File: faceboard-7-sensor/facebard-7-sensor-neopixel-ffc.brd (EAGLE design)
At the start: 26 x 93.5 mm, 32 parts, among them Q1 QRE1113, Q2 QRE1113, Q3 QRE1113, Q4 QRE1113, Q5 QRE1113, Q6 QRE1113, Q7 QRE1113, U1 CD4051BE

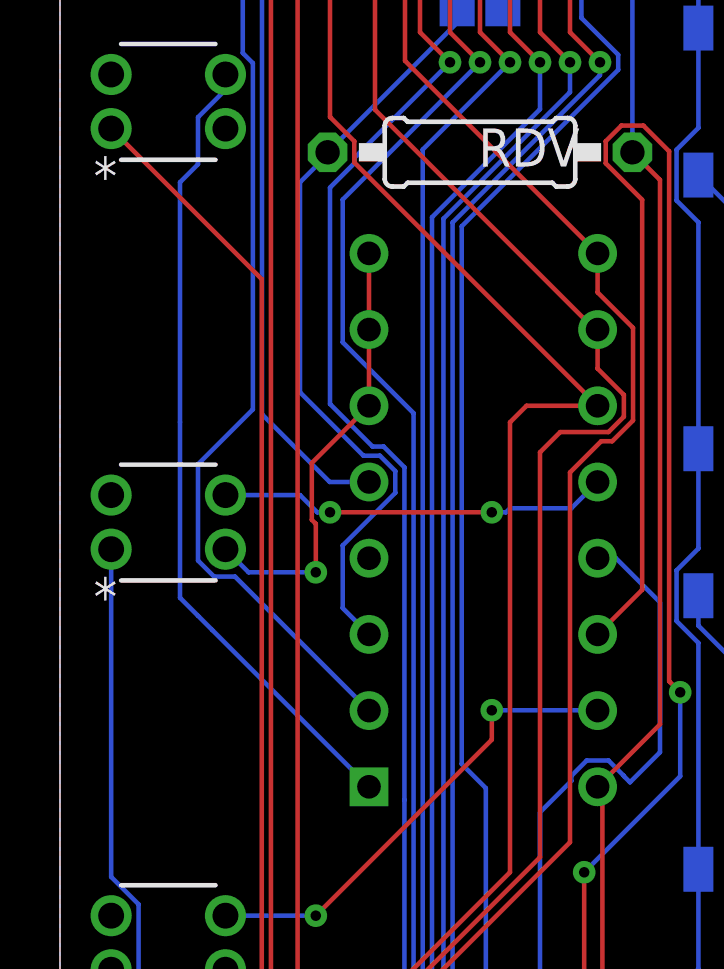
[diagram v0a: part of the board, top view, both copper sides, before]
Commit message: tidy routing
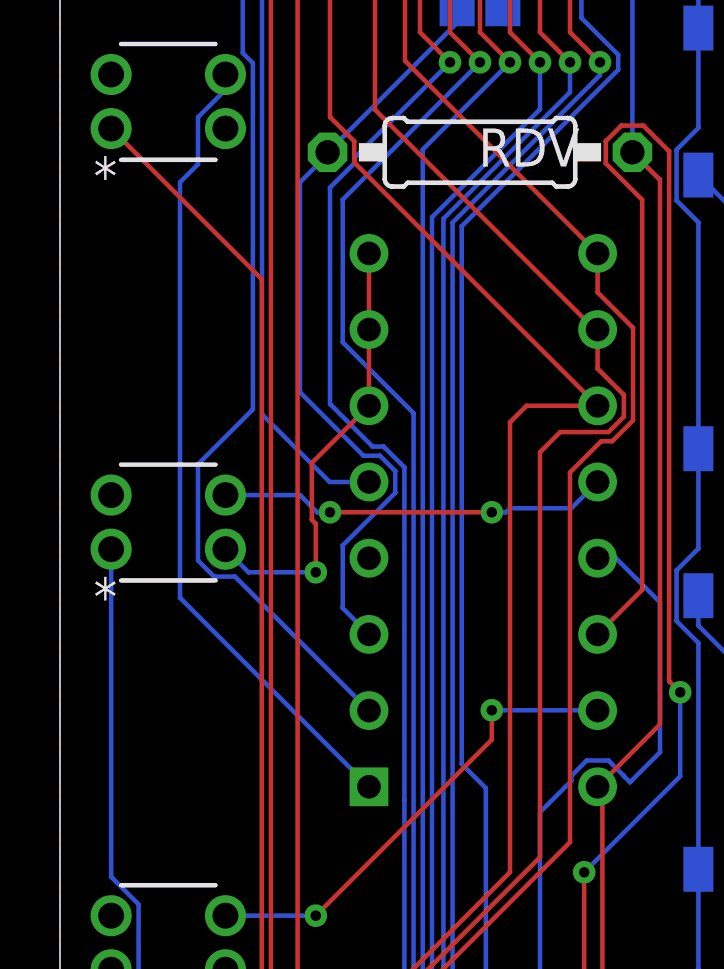
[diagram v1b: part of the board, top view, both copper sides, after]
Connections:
- net Q1SIG renamed C0
- net Q2SIG renamed C1
- net Q3SIG renamed C2
- net Q4SIG renamed C3
- net Q5SIG renamed C4
- net Q6SIG renamed C5
- net Q7SIG renamed C6
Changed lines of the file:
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@@
 <wire x1="6.7" y1="15.7" x2="7.92" y2="15.7" width="0.1524" layer="1"/>
 </signal>
-<signal name="Q1SIG">
+<signal name="C0">
 <contactref element="U1" pad="13"/>
-<contactref element="Q1" pad="3"/>
-<wire x1="5.515" y1="5.5134" x2="5.515" y2="12.515" width="0.1524" layer="16"/>
 <wire x1="5.515" y1="12.515" x2="7" y2="14" width="0.1524" layer="16"/>
 <wire x1="7" y1="14" x2="11" y2="14" width="0.1524" layer="16"/>
@@
 <wire x1="20" y1="39" x2="20" y2="44" width="0.1524" layer="16"/>
 <wire x1="20" y1="44" x2="18.53" y2="45.47" width="0.1524" layer="16"/>
+<contactref element="Q1" pad="3"/>
+<wire x1="5.515" y1="5.5134" x2="5.515" y2="12.515" width="0.1524" layer="16"/>
 </signal>
 <signal name="GND">
@@
 <wire x1="6.5356" y1="16.8156" x2="7.92" y2="18.2" width="0.1524" layer="1"/>
 </signal>
-<signal name="Q2SIG">
-<contactref element="Q2" pad="3"/>
+<signal name="C1">
 <contactref element="U1" pad="14"/>
 <via x="11" y="20.4334" extent="1-16" drill="0.35"/>
@@
 <wire x1="20.3048" y1="41.3684" x2="20.3048" y2="59.0324375" width="0.1524" layer="1"/>
 <wire x1="20.3048" y1="59.0324375" x2="19.4482375" y2="59.889" width="0.1524" layer="1"/>
+<wire x1="10.1" y1="19.5334" x2="11" y2="20.4334" width="0.1524" layer="16"/>
+<contactref element="Q2" pad="3"/>
 <wire x1="5.515" y1="19.5334" x2="10.1" y2="19.5334" width="0.1524" layer="16"/>
-<wire x1="10.1" y1="19.5334" x2="11" y2="20.4334" width="0.1524" layer="16"/>
 </signal>
 <signal name="N$5">
@@
 <wire x1="6.0922" y1="27.073725" x2="1.705" y2="31.460925" width="0.1524" layer="1"/>
 </signal>
-<signal name="Q3SIG">
-<contactref element="Q3" pad="3"/>
+<signal name="C2">
 <contactref element="U1" pad="15"/>
-<wire x1="5.515" y1="33.5534" x2="8.5268" y2="33.5534" width="0.1524" layer="16"/>
 <via x="8.5268" y="33.5534" extent="1-16" drill="0.35"/>
 <wire x1="8.5268" y1="33.5534" x2="14.3932" y2="39.4198" width="0.1524" layer="1"/>
@@
 <wire x1="14.3932" y1="40.4" x2="17.91" y2="40.4" width="0.1524" layer="16"/>
 <wire x1="17.91" y1="40.4" x2="17.92" y2="40.39" width="0.1524" layer="16"/>
+<contactref element="Q3" pad="3"/>
+<wire x1="5.515" y1="33.5534" x2="8.5268" y2="33.5534" width="0.1524" layer="16"/>
 </signal>
 <signal name="N$7">
@@
 <wire x1="2.6194" y1="30.546525" x2="2.6194" y2="33.9321625" width="0.1524" layer="16"/>
 </signal>
-<signal name="Q4SIG">
-<contactref element="Q4" pad="3"/>
+<signal name="C3">
 <contactref element="U1" pad="12"/>
-<wire x1="5.515" y1="47.5734" x2="8" y2="47.5734" width="0.1524" layer="16"/>
 <wire x1="15" y1="47.1337" x2="17.0437" y2="47.1337" width="0.1524" layer="16"/>
 <wire x1="17.0437" y1="47.1337" x2="17.92" y2="48.01" width="0.1524" layer="16"/>
-<wire x1="8" y1="47.5734" x2="8.5734" y2="47" width="0.1524" layer="16"/>
+<wire x1="8.0267" y1="47.5467" x2="8.5734" y2="47" width="0.1524" layer="16"/>
 <wire x1="8.5734" y1="47" x2="9" y2="47" width="0.1524" layer="16"/>
 <via x="9" y="47" extent="1-16" drill="0.35"/>
@@
 <wire x1="15" y1="47.1337" x2="14.8663" y2="47" width="0.1524" layer="16"/>
 <wire x1="9" y1="47" x2="14.3932" y2="47" width="0.1524" layer="1"/>
+<contactref element="Q4" pad="3"/>
+<wire x1="5.515" y1="47.5734" x2="8" y2="47.5734" width="0.1524" layer="16"/>
+<wire x1="8" y1="47.5734" x2="8.0267" y2="47.5467" width="0.1524" layer="16"/>
 </signal>
 <signal name="N$9">
@@
 <wire x1="6.7262" y1="27.2365625" x2="6.7262" y2="54.7688" width="0.1524" layer="1"/>
 </signal>
-<signal name="Q5SIG">
-<contactref element="Q5" pad="3"/>
+<signal name="C4">
 <contactref element="U1" pad="1"/>
-<wire x1="4.6006" y1="43.5494" x2="5.075" y2="43.075" width="0.1524" layer="16"/>
-<wire x1="5.075" y1="43.075" x2="10.3" y2="37.85" width="0.1524" layer="16"/>
-<wire x1="5.515" y1="61.5934" x2="5.515" y2="61.0831625" width="0.1524" layer="16"/>
+<wire x1="4" y1="44.15" x2="10.3" y2="37.85" width="0.1524" layer="16"/>
 <wire x1="4.6006" y1="58.6006" x2="4" y2="58" width="0.1524" layer="16"/>
 <wire x1="5.515" y1="61.0831625" x2="4.6006" y2="60.1687625" width="0.1524" layer="16"/>
 <wire x1="4.6006" y1="60.1687625" x2="4.6006" y2="58.6006" width="0.1524" layer="16"/>
-<wire x1="4" y1="58" x2="4" y2="50" width="0.1524" layer="16"/>
-<wire x1="4" y1="50" x2="4" y2="44.15" width="0.1524" layer="16"/>
-<wire x1="4" y1="44.15" x2="4.6006" y2="43.5494" width="0.1524" layer="16"/>
+<wire x1="4" y1="58" x2="4" y2="44.15" width="0.1524" layer="16"/>
+<contactref element="Q5" pad="3"/>
+<wire x1="5.515" y1="61.5934" x2="5.515" y2="61.0831625" width="0.1524" layer="16"/>
 </signal>
 <signal name="N$11">
@@
 <wire x1="7.031" y1="29.6317625" x2="7.031" y2="68.484" width="0.1524" layer="1"/>
 </signal>
-<signal name="Q6SIG">
-<contactref element="Q6" pad="3"/>
+<signal name="C5">
 <contactref element="U1" pad="5"/>
-<wire x1="5.515" y1="75.6134" x2="5.515" y2="75.1031625" width="0.1524" layer="16"/>
 <wire x1="5.515" y1="75.1031625" x2="6.7342" y2="73.8839625" width="0.1524" layer="16"/>
 <wire x1="6.7342" y1="73.8839625" x2="6.7342" y2="50.2658" width="0.1524" layer="16"/>
 <wire x1="8.99" y1="48.01" x2="10.3" y2="48.01" width="0.1524" layer="16"/>
 <wire x1="6.7342" y1="50.2658" x2="8.99" y2="48.01" width="0.1524" layer="16"/>
+<contactref element="Q6" pad="3"/>
+<wire x1="5.515" y1="75.6134" x2="5.515" y2="75.1031625" width="0.1524" layer="16"/>
 </signal>
 <signal name="N$13">
@@
 <wire x1="7.92" y1="75.08" x2="1.705" y2="81.295" width="0.1524" layer="1"/>
 </signal>
-<signal name="Q7SIG">
-<contactref element="Q7" pad="3"/>
+<signal name="C6">
 <contactref element="U1" pad="2"/>
 <wire x1="6.4294" y1="88.2087625" x2="6.4294" y2="87.4512375" width="0.1524" layer="16"/>
-<wire x1="5.515" y1="89.6334" x2="5.515" y2="89.1231625" width="0.1524" layer="16"/>
 <wire x1="5.515" y1="89.1231625" x2="6.4294" y2="88.2087625" width="0.1524" layer="16"/>
 <wire x1="4.6006" y1="73.4312375" x2="5" y2="73.0318375" width="0.1524" layer="16"/>
@@
 <wire x1="4.6006" y1="48.6006" x2="4.6006" y2="45.3912375" width="0.1524" layer="16"/>
 <wire x1="6.4294" y1="50.4294" x2="4.6006" y2="48.6006" width="0.1524" layer="16"/>
+<contactref element="Q7" pad="3"/>
+<wire x1="5.515" y1="89.6334" x2="5.515" y2="89.1231625" width="0.1524" layer="16"/>
 </signal>
 <signal name="SIG">
